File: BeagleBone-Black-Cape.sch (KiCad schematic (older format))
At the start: 2 parts, among them P101 BeagleBone_Black_Header, P102 BeagleBone_Black_Header

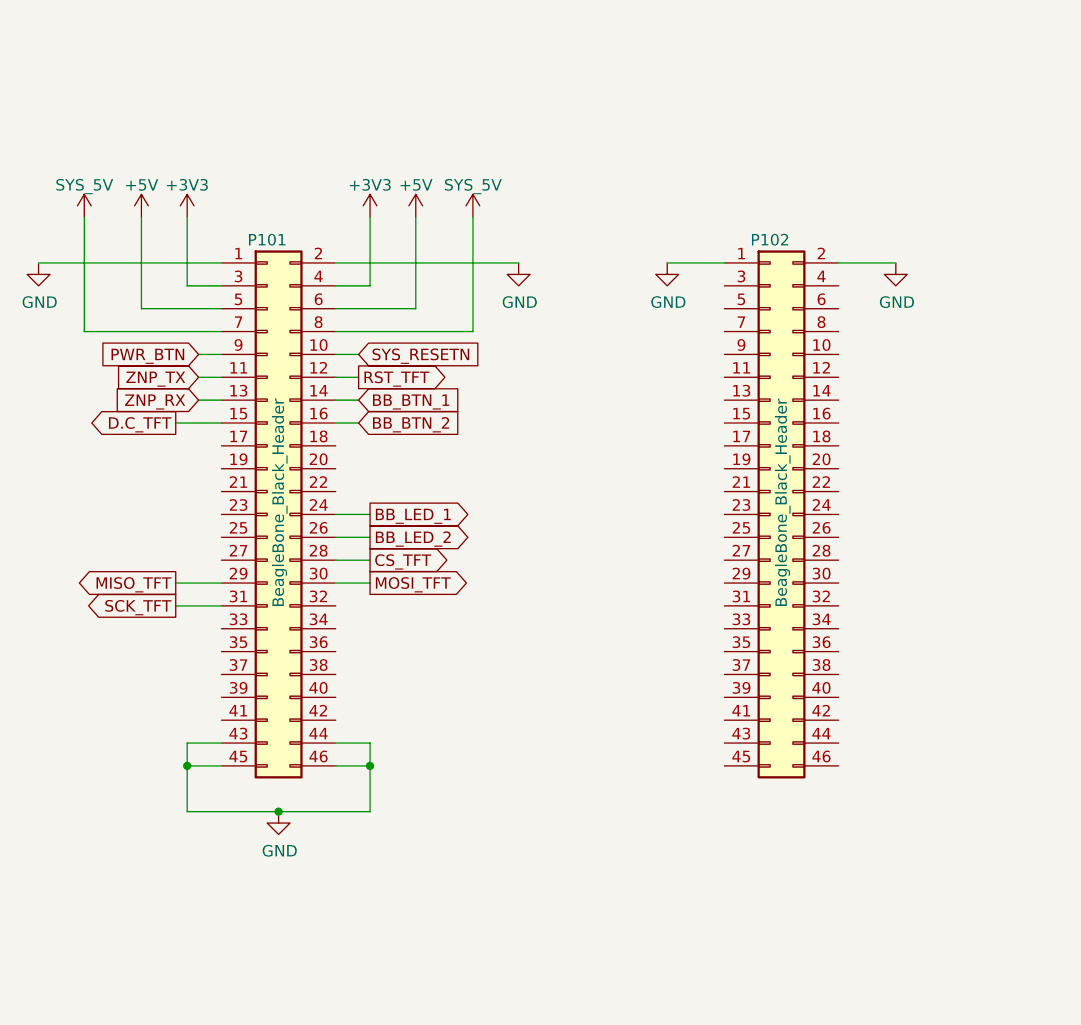
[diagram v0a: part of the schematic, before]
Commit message: sync push so zach can work
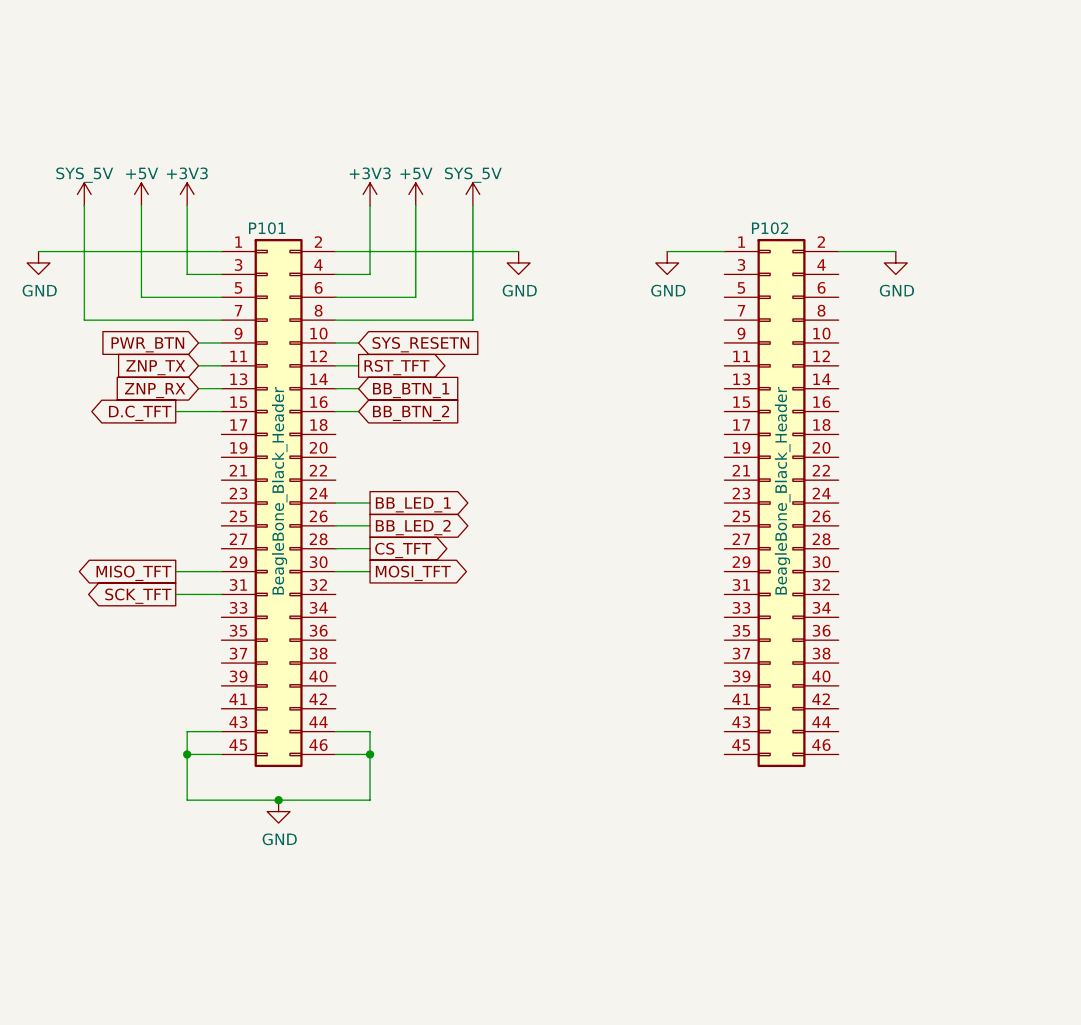
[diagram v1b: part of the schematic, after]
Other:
- moved on the sheet: P101, P102
